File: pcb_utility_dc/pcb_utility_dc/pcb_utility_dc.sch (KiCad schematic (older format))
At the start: 1 part

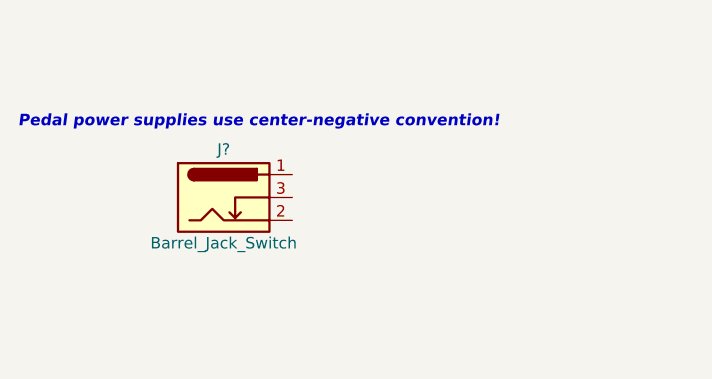
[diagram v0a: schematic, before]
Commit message: Start schematic and layout
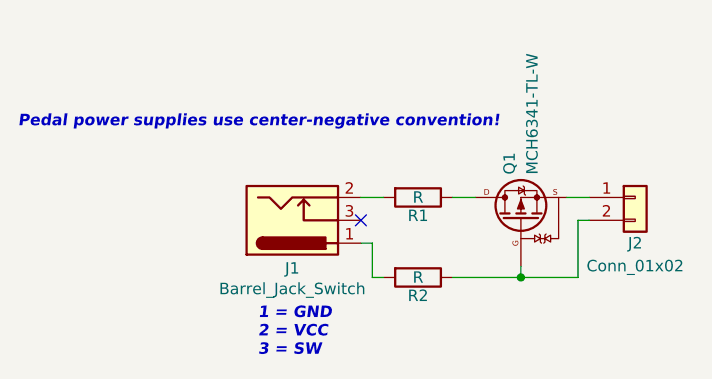
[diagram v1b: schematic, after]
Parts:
- added J2: Conn_01x02, Connector_Wire:SolderWirePad_1x02_P3.81mm_Drill0.8mm, symbol Connector_Generic:Conn_01x02
- added Q1: MCH6341-TL-W, Transistors_MOSFETS_SMD:ON_Semi_MCH6341-TL-W, symbol Transistors_MOSFETS_SMD:MCH6341-TL-W
- added R1, R2: R, Resistor_SMD:R_0603_1608Metric, symbol Device:R
- J1: renamed from J?; footprint (none) -> Connectors_Jacks_DC:Jack_DC
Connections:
- net at J1.1: now also R2.2
- net at J1.2: now also R1.2
- new net: Q1.D, R1.1
- new net: J2.2 (Pin_2), Q1.G, R2.1
- new net: J2.1 (Pin_1), Q1.S
- no-connect marks 0 -> 1
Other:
- note added: "1 = GND\n2 = VCC\n3 = SW"
- moved on the sheet: J1
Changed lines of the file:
@@
 $EndDescr
 $Comp
-L Connector:Barrel_Jack_Switch J?
+L Connector:Barrel_Jack_Switch J1
 U 1 1 5BFAD889
-P 5400 3900
-F 0 "J?" H 5400 4110 50  0000 C CNN
-F 1 "Barrel_Jack_Switch" H 5400 3700 50  0000 C CNN
-F 2 "" H 5450 3860 50  0001 C CNN
-F 3 "~" H 5450 3860 50  0001 C CNN
-	1    5400 3900
-	1    0    0    -1
+P 5700 4000
+F 0 "J1" H 5700 4210 50  0000 C CNN
+F 1 "Barrel_Jack_Switch" H 5700 4300 50  0000 C CNN
+F 2 "Connectors_Jacks_DC:Jack_DC" H 5750 3960 50  0001 C CNN
+F 3 "~" H 5750 3960 50  0001 C CNN
+	1    5700 4000
+	1    0    0    1
 $EndComp
 Text Notes 4500 3600 0    50   Italic 10
 Pedal power supplies use center-negative convention!
+$Comp
+L Transistors_MOSFETS_SMD:MCH6341-TL-W Q1
+U 1 1 5BFAE35A
+P 6700 4000
+F 0 "Q1" H 6900 4050 50  0000 L CNN
+F 1 "MCH6341-TL-W" H 6900 3950 50  0000 L CNN
+F 2 "Transistors_MOSFETS_SMD:ON_Semi_MCH6341-TL-W" H 6900 4100 50  0001 C CNN
+F 3 "~" H 6700 4000 50  0001 C CNN
+	1    6700 4000
+	0    -1   -1   0
+$EndComp
+$Comp
+L Device:R R1
+U 1 1 5BFB200F
+P 6250 3900
+F 0 "R1" V 6330 3900 50  0000 C CNN
+F 1 "R" V 6250 3900 50  0000 C CNN
+F 2 "Resistor_SMD:R_0603_1608Metric" V 6180 3900 50  0001 C CNN
+F 3 "~" H 6250 3900 50  0001 C CNN
+	1    6250 3900
+	0    1    1    0
+$EndComp
+Wire Wire Line
+	6500 3900 6400 3900
+Wire Wire Line
+	6100 3900 6000 3900
+Wire Wire Line
+	6700 4200 6700 4250
+$Comp
+L Connector_Generic:Conn_01x02 J2
+U 1 1 5BFB32FD
+P 7200 3900
+F 0 "J2" H 7200 3700 50  0000 C CNN
+F 1 "Conn_01x02" H 7200 3600 50  0000 C CNN
+F 2 "Connector_Wire:SolderWirePad_1x02_P3.81mm_Drill0.8mm" H 7200 3900 50  0001 C CNN
+F 3 "~" H 7200 3900 50  0001 C CNN
+	1    7200 3900
+	1    0    0    -1
+$EndComp
+Wire Wire Line
+	7000 3900 6900 3900
+Wire Wire Line
+	7000 4000 6950 4000
+Text Notes 5550 4600 0    50   Italic 10
+1 = GND\n2 = VCC\n3 = SW
+$Comp
+L Device:R R2
+U 1 1 5BFB4BDE
+P 6250 4250
+F 0 "R2" V 6330 4250 50  0000 C CNN
+F 1 "R" V 6250 4250 50  0000 C CNN
+F 2 "Resistor_SMD:R_0603_1608Metric" V 6180 4250 50  0001 C CNN
+F 3 "~" H 6250 4250 50  0001 C CNN
+	1    6250 4250
+	0    1    1    0
+$EndComp
+Wire Wire Line
+	6400 4250 6700 4250
+Wire Wire Line
+	6100 4250 6050 4250
+Wire Wire Line
+	6050 4250 6050 4100
+Wire Wire Line
+	6050 4100 6000 4100
+Wire Wire Line
+	6700 4250 6950 4250
+Wire Wire Line
+	6950 4250 6950 4000
+Connection ~ 6700 4250
+NoConn ~ 6000 4000
 $EndSCHEMATC

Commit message: us8 based switching files
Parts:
- J1: footprint Connectors_Jacks_DC:Jack_DC -> Connectors_Jacks_DC:Jack_DC_Mirrored
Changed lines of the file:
@@
 EESchema Schematic File Version 4
+LIBS:pcb_utility_dc-cache
 EELAYER 29 0
 EELAYER END
@@
 F 0 "J1" H 5700 4210 50  0000 C CNN
 F 1 "Barrel_Jack_Switch" H 5700 4300 50  0000 C CNN
-F 2 "Connectors_Jacks_DC:Jack_DC" H 5750 3960 50  0001 C CNN
+F 2 "Connectors_Jacks_DC:Jack_DC_Mirrored" H 5750 3960 50  0001 C CNN
 F 3 "~" H 5750 3960 50  0001 C CNN
 	1    5700 4000
